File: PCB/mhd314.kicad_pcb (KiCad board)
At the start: 4 copper layers, 65 x 56 mm, 201 parts, among them J1 Raspberry_Pi_2_3, J2 AudioJack_Pentaconn, J4 AudioJack3_SwitchTR, Q1 AO3401A, SW1 SW_Push, U1 ES9038Q2M, U10 AT24CS64-SSHM, U11 OPA1622, U13 OPA1622, U2 OPA1612AxD, U3 OPA1612AxD, U4 OPA1622, U5 LM317_SOT-223, U6 LM317_SOT-223, U7 TPS65131RGE, U8 LM317_SOT-223, U9 LM337_SOT223, Y1 ASE-50MHz

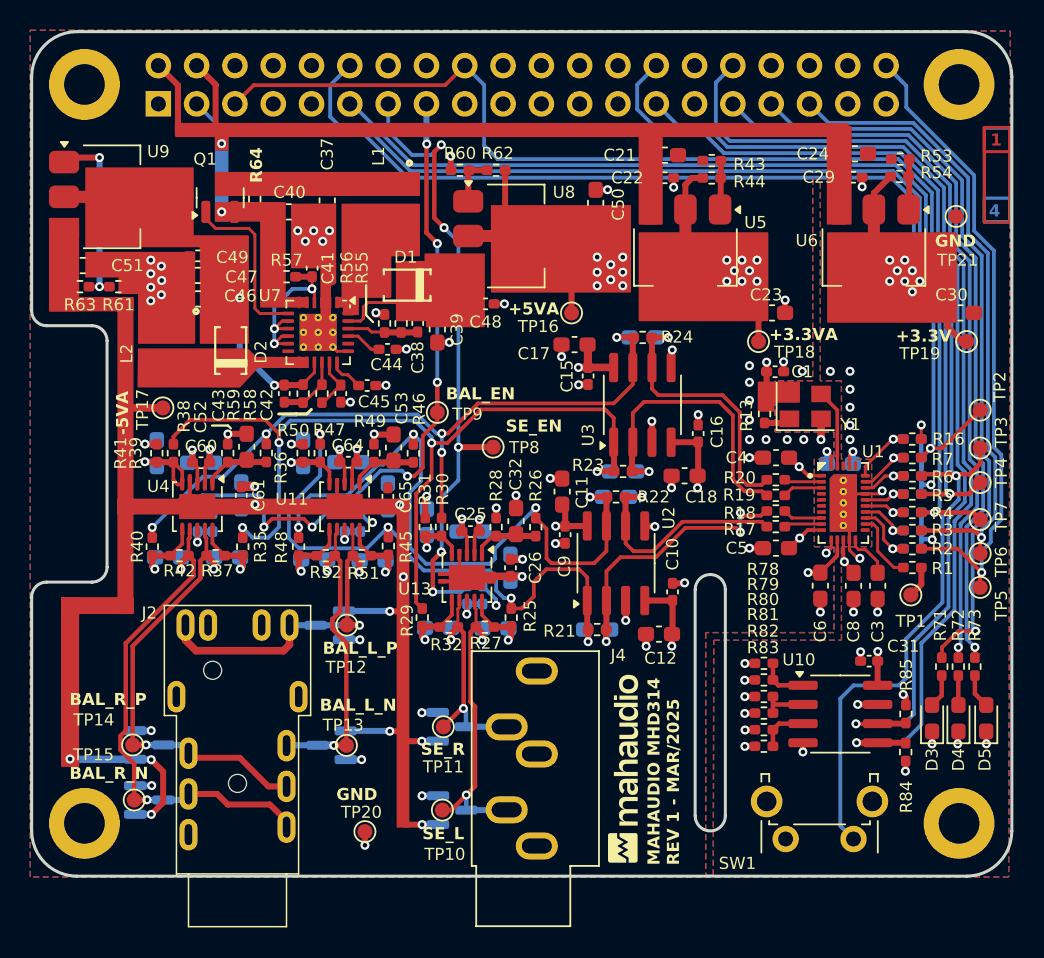
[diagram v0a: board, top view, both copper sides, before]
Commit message: Redone placement and layout of OPA1622. Still finishing touches
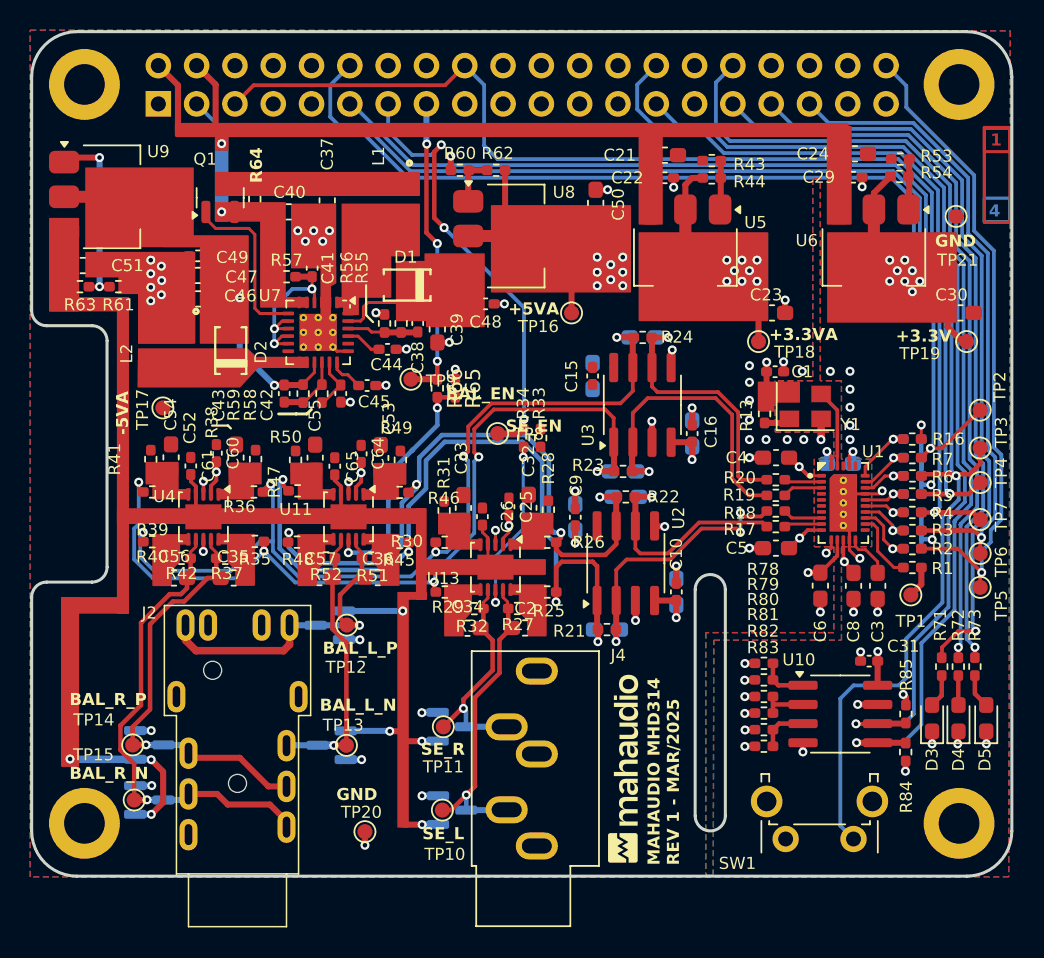
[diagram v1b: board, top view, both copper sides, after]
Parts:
- removed C27, C28, C62, C63, C66, C67: 1uF, Capacitor_SMD:C_0603_1608Metric_Pad1.08x0.95mm_HandSolder
- removed R74, R76: 10k, Resistor_SMD:R_0402_1005Metric_Pad0.72x0.64mm_HandSolder
- removed R75, R77: 22R, Resistor_SMD:R_0402_1005Metric_Pad0.72x0.64mm_HandSolder
- added R65: 10k, Resistor_SMD:R_0402_1005Metric_Pad0.72x0.64mm_HandSolder, F.Cu at (128.2, 67.6)
- added R66: 22R, Resistor_SMD:R_0402_1005Metric_Pad0.72x0.64mm_HandSolder, F.Cu at (127.0, 67.6)
- C11, C12, C17, C18: moved to B.Cu
- C2, C33, C34, C35, C36, C54, C55, C56, C57, R33, R34: moved to F.Cu
- moved R33 11.1 mm to (133.8, 70.9)
- moved R34 11.1 mm to (132.7, 70.9)
- moved C65 4.05 mm to (120.2, 72.8)
- moved C61 3.88 mm to (110.7, 72.8)
- moved C26 3.87 mm to (130.0, 76.1)
- moved R28 3.65 mm to (134.4, 75.7)
- moved C25 3.04 mm to (131.8, 75.5), turned to 90 degrees
- moved C12 3.03 mm to (142.8, 81.1), turned to -90 degrees
- moved R39 2.93 mm to (108.1, 74.5), turned to 0 degrees
- moved R25 2.93 mm to (134.3, 81.1), turned to 180 degrees
- moved R47 2.92 mm to (117.7, 74.4), turned to 0 degrees
- moved C18 2.84 mm to (143.9, 70.6), turned to -90 degrees
- moved TP9 2.81 mm to (125.2, 67.0)
- moved R46 2.75 mm to (124.5, 74.5), turned to 180 degrees
- moved R36 2.71 mm to (114.8, 74.5), turned to 180 degrees
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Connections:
- U11 pad 8: Net-(U11A-EN) -> /AMP/BalDiffAmp_L/BALDIFFAMP_ENABLE
- U4 pad 8: Net-(U4A-EN) -> /AMP/BalDiffAmp_L/BALDIFFAMP_ENABLE
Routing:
- net /AMP/BalDiffAmp_L/BALDIFFAMP_ENABLE: track 0.00 -> 27.3 mm, vias 0 -> 3
- net /AMP_DIFF_EN: track 45.5 -> 20.3 mm, vias 6 -> 3
- net GND: track 77.8 -> 53.0 mm, vias 87 -> 72
- net /AMP_SE_EN: track 42.3 -> 29.8 mm, vias 5 -> 3
- net +5VA: track 41.7 -> 29.8 mm, vias 19 -> 18
- net /AMP/BalDiffAmp_L/BALDIFFAMP_IN_P: track 40.3 -> 52.0 mm
- net Net-(U13A-EN): track 2.68 -> 11.9 mm, vias 1 -> 2
- net /AMP/BalDiffAmp_R/BALDIFFAMP_IN_N: track 49.7 -> 57.7 mm
- net -5VA: track 46.4 -> 38.6 mm, vias 13 -> 9
- net Net-(U11A--): track 6.28 -> 0.00 mm, vias 1 -> 0
- net Net-(U4B-+): track 6.18 -> 0.00 mm, vias 1 -> 0
- net Net-(U13B--): track 6.07 -> 0.00 mm, vias 1 -> 0
- net Net-(U11B--): track 5.45 -> 0.00 mm, vias 1 -> 0
- net Net-(U4A--): track 5.41 -> 0.00 mm, vias 1 -> 0
- net Net-(U13B-+): track 5.40 -> 0.00 mm, vias 1 -> 0
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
